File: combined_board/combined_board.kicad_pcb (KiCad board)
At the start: 2 copper layers, 131.9 x 83.5 mm, 62 parts, among them IC1 SN74LVC1G3157DBVR, IC2 AD8542ARMZ-REEL, IC3 SN74LVC1G3157DBVR, J1 PINHD_1x2_Male, J10 USB4736, J11 Conn_01x25_Pin, J12 Conn_01x25_Pin, J13 Conn_01x02_Pin, J14 PINHD_1x2_Male, J14_GND1 Conn_01x03, J14_GND2 Conn_01x03, J2 PINHD_1x2_Male, J3 PINHD_1x2_Male, J6 PINHD_1x2_Male, J7 PINHD_1x2_Male, J8 Conn_01x25_Pin, J9 Conn_01x25_Pin, U1 NCV8164ASN250T1G_LDO_2.5V

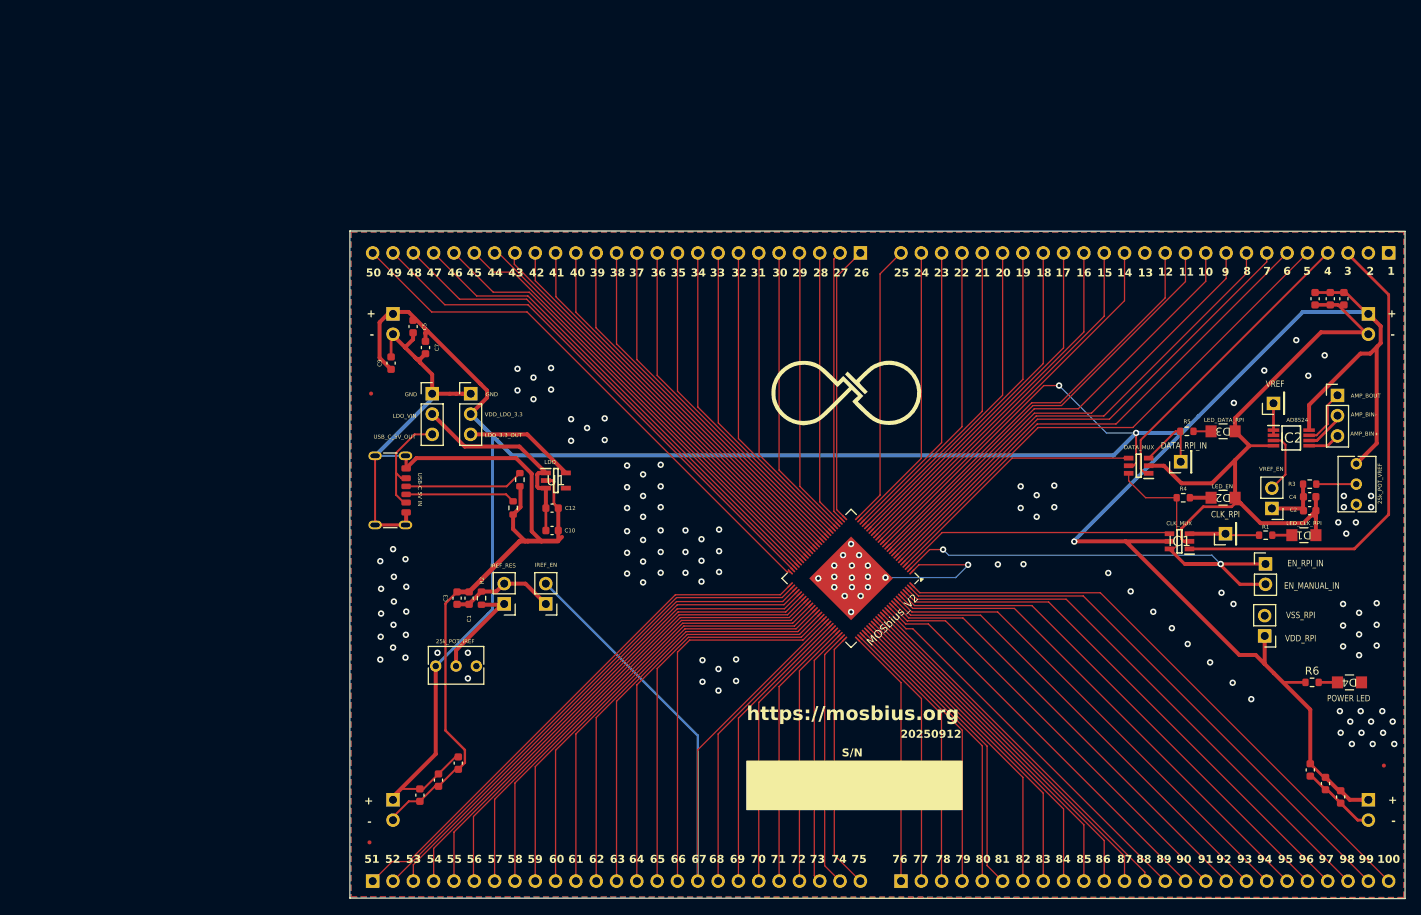
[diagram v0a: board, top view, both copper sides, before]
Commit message: 0311_2026 XP update - mainly in RPI board
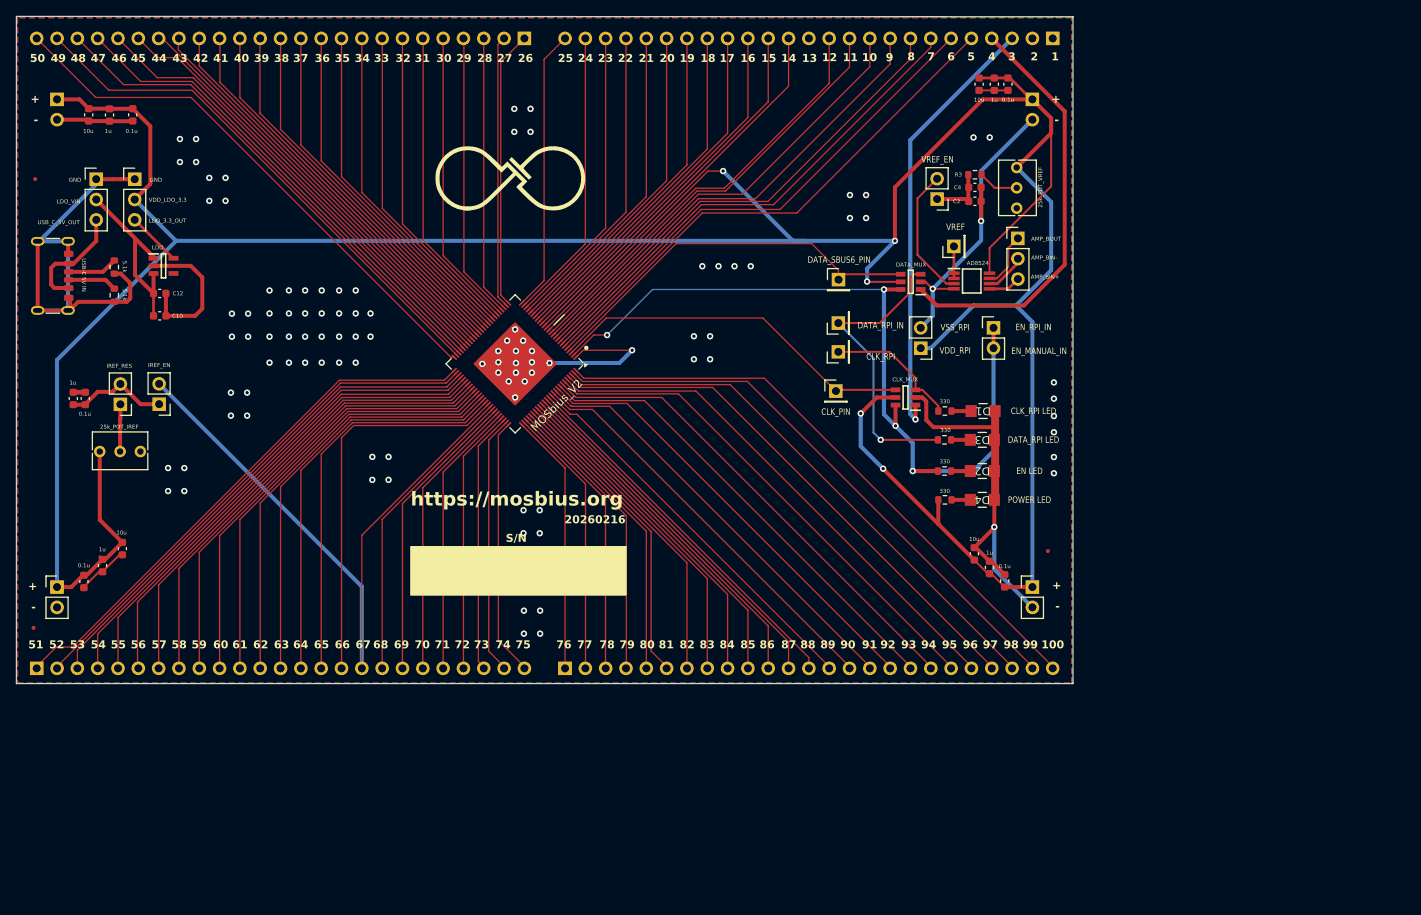
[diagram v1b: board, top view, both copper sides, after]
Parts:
- removed R2: 1k, Resistor_SMD:R_0603_1608Metric
- added J_VCM2: DIRECT_DATA_SBUS, Connector_PinHeader_2.54mm:PinHeader_1x01_P2.54mm_Vertical, F.Cu at (147.1, 61.8)
- added J_VCM3: DIRECT_CLK, Connector_PinHeader_2.54mm:PinHeader_1x01_P2.54mm_Vertical, F.Cu at (146.8, 75.7)
- J14, J7: moved to F.Cu
- moved Rd_1 57.2 mm to (56.6, 60.2)
- moved C2 57.0 mm to (164.2, 52.0)
- moved C4 57.0 mm to (164.2, 50.2)
- moved R3 57.0 mm to (164.2, 48.6)
- moved J2 57.0 mm to (159.5, 51.7)
- moved Rd_2 56.5 mm to (56.6, 63.7)
- moved RV2 56.3 mm to (169.4, 47.7)
- moved VDD_GND_RPI1 56.1 mm to (157.4, 70.3)
- moved C10 55.9 mm to (62.3, 66.3)
- moved C12 55.9 mm to (62.3, 63.5)
- moved U1 55.9 mm to (62.8, 60.0)
- moved J1 54.4 mm to (62.2, 77.3)
- moved C1 54.1 mm to (53.0, 76.6)
- moved C3 54.1 mm to (51.5, 76.6)
- moved J3 54.1 mm to (57.4, 77.3)
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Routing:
- net GND: track 263.1 -> 207.8 mm, vias 131 -> 103
- net VDD: track 395.4 -> 428.6 mm, vias 3 -> 5
- net Net-(IC3-B1): track 9.48 -> 37.8 mm, vias 0 -> 1
- net /EN: track 79.5 -> 101.3 mm, vias 2 -> 4
- net /DATA_SBUS6: track 34.1 -> 49.8 mm
- net /SBUS6: track 37.9 -> 53.0 mm
- net /CLK: track 34.6 -> 46.8 mm
- net Net-(IC2-+IN_A): track 7.85 -> 16.6 mm
- net Net-(J10-CC1): track 14.9 -> 6.29 mm
- net Net-(IC1-B1): track 8.97 -> 16.8 mm
- net Net-(J10-CC2): track 13.7 -> 6.16 mm
- net Net-(J3-Pad1): track 13.3 -> 6.07 mm
- net LDO_OUT_3.3V: track 14.6 -> 7.55 mm
- net /CLK_SC: track 61.9 -> 55.0 mm, vias 0 -> 1
- net LDO_VIN: track 27.3 -> 24.4 mm
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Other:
- board size 131.9 x 83.5 mm -> 132.1 x 83.4 mm
- board text added: "0.1u"
- board text added: "10u"
- board text added: "1u"
- board text added: "20260216"
- board text added: "330"
- board text added: "5.1k"
- board text added: "CLK_PIN"
- board text added: "CLK_RPI LED"
- board text added: "DATA_RPI LED"
- board text added: "DATA_SBUS6_PIN"
- board text added: "EN LED"
- board text removed: "127mm"
- board text removed: "20250912"
- board text removed: "34.4mm"
- board text removed: "5.08mm (2 blocks on breadboard)"
- board text removed: "7.62mm (3 blocks on breadboard)"
- board text removed: "78.5mm"
- board text removed: "LED_CLK_RPI"
- board text removed: "LED_DATA_RPI"
- board text removed: "LED_EN"
